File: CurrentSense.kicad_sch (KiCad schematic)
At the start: 4 parts, among them J3 XT60PW-M, U4 INA181A3IDBVR

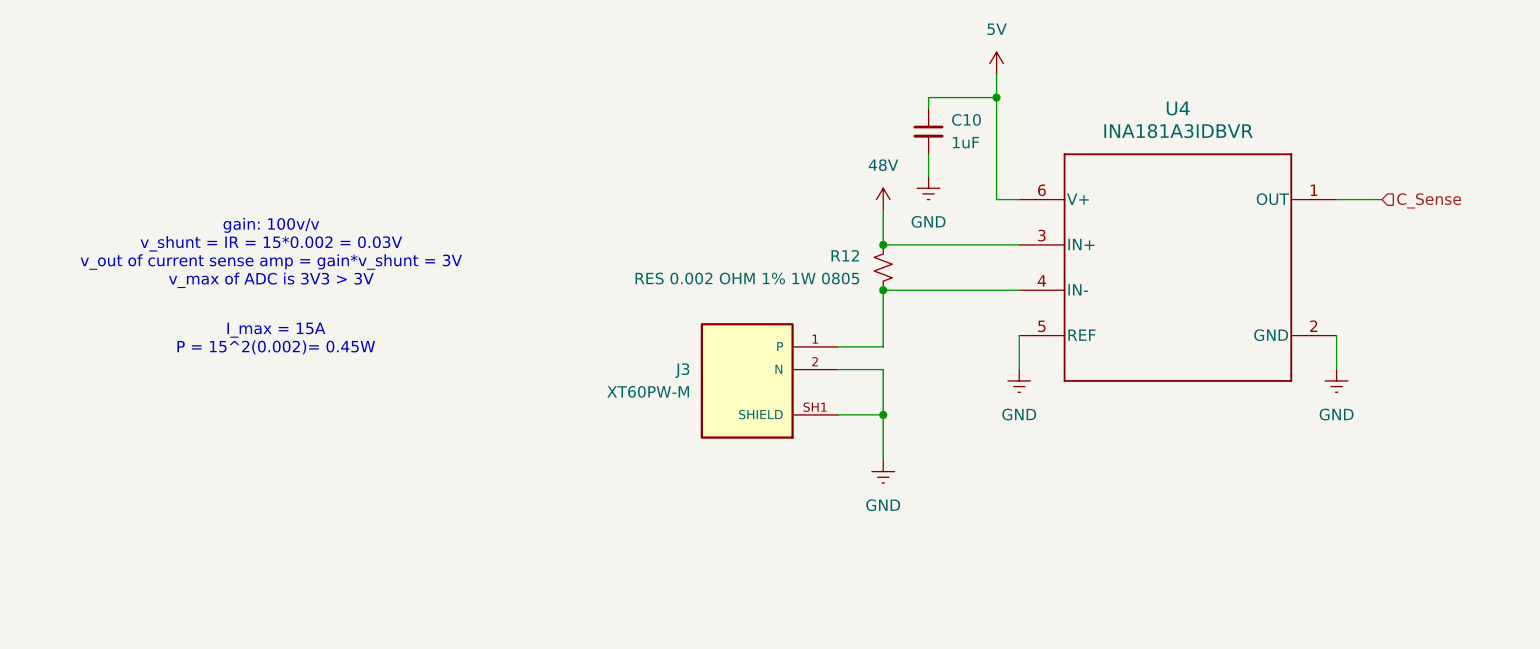
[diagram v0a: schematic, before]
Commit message: damir review
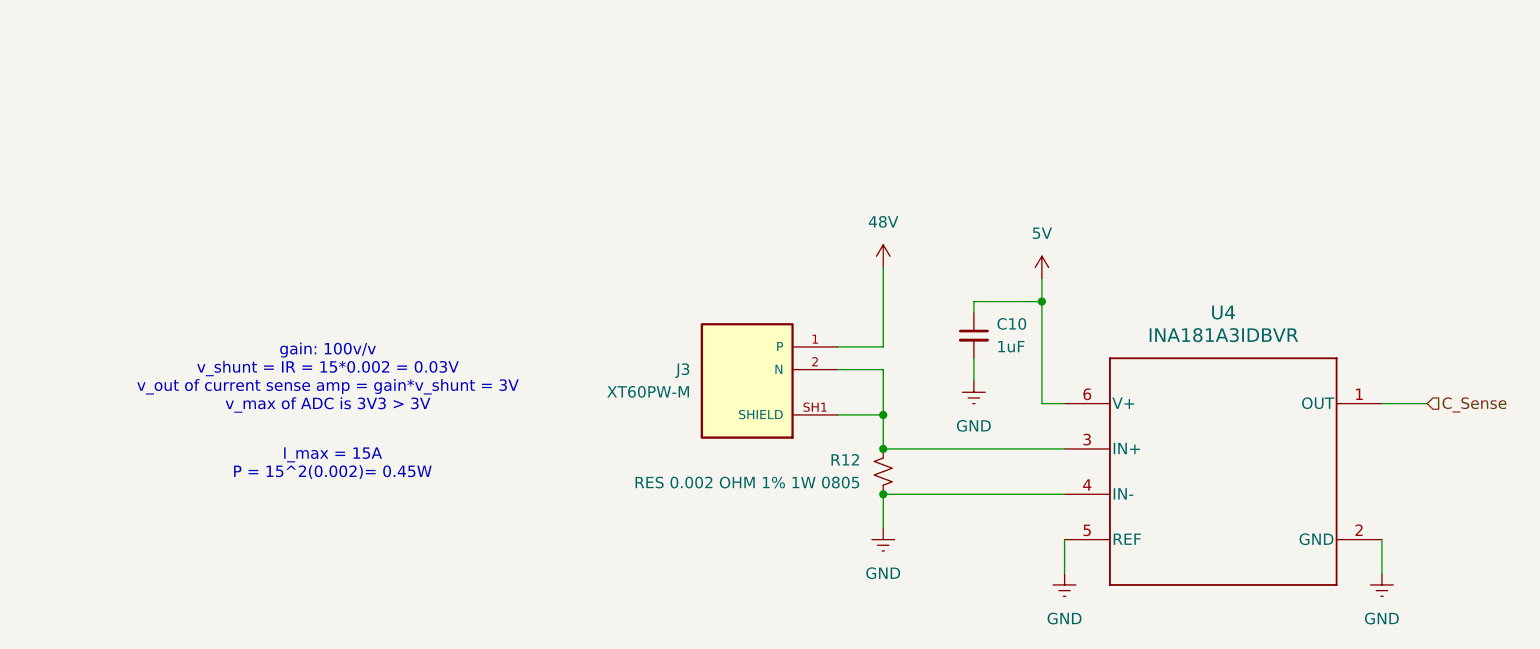
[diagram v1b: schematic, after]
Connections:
- net 48V: now also J3.1 (P); no longer R12.1, U4.3 (IN+)
- net GND: now also R12.2, U4.4 (IN-); no longer J3.2 (N), J3.SH1 (SHIELD), J3.SH2 (SHIELD)
- new net: J3.2 (N), J3.SH1 (SHIELD), J3.SH2 (SHIELD), R12.1, U4.3 (IN+)
